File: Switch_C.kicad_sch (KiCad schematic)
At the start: 2 parts

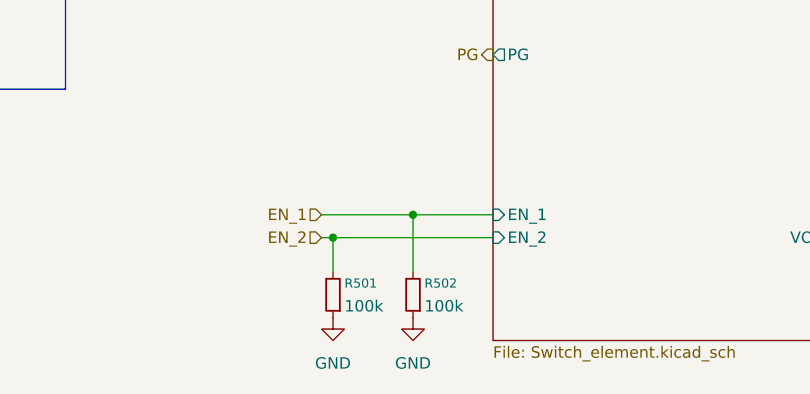
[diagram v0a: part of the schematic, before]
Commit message: small changes to test board
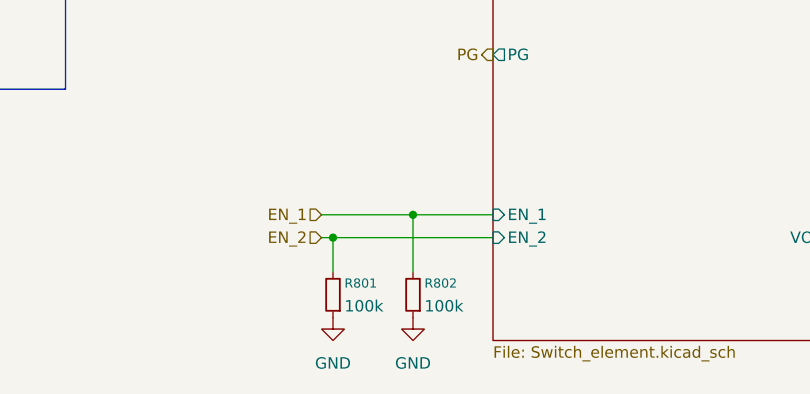
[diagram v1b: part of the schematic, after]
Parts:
- renumbered R501 to R801, R502 to R802
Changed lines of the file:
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@@
 		(on_board yes)
 		(dnp no)
-		(property "Reference" "R501"
+		(property "Reference" "R801"
 			(at 96.52 121.92 0)
 			(effects
@@
 		(on_board yes)
 		(dnp no)
-		(property "Reference" "R502"
+		(property "Reference" "R802"
 			(at 105.41 121.92 0)
 			(effects
@@
 		(dnp no)
 		(fields_autoplaced yes)
-		(property "Reference" "#PWR0164"
+		(property "Reference" "#PWR0165"
 			(at 95.25 132.08 0)
 			(effects
@@
 		(dnp no)
 		(fields_autoplaced yes)
-		(property "Reference" "#PWR0165"
+		(property "Reference" "#PWR0166"
 			(at 104.14 132.08 0)
 			(effects

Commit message: nearly finnished CORE pcb
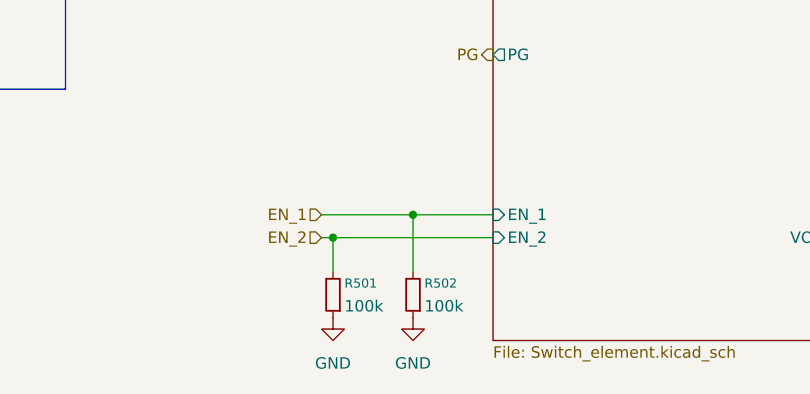
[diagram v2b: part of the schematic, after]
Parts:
- renumbered R801 to R501, R802 to R502
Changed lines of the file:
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@@
 		(on_board yes)
 		(dnp no)
-		(property "Reference" "R801"
+		(property "Reference" "R501"
 			(at 96.52 121.92 0)
 			(effects
@@
 		(on_board yes)
 		(dnp no)
-		(property "Reference" "R802"
+		(property "Reference" "R502"
 			(at 105.41 121.92 0)
 			(effects
@@
 		(dnp no)
 		(fields_autoplaced yes)
-		(property "Reference" "#PWR0165"
+		(property "Reference" "#PWR0164"
 			(at 95.25 132.08 0)
 			(effects
@@
 		(dnp no)
 		(fields_autoplaced yes)
-		(property "Reference" "#PWR0166"
+		(property "Reference" "#PWR0165"
 			(at 104.14 132.08 0)
 			(effects
